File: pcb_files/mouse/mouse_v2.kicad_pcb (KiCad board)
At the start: 2 copper layers, 84.9 x 94.9 mm, 58 parts, among them J4 I2C_Conn, M1 Motor_DC, M2 Motor_DC, Q0 Q_Photo_NPN, Q1 Q_Photo_NPN, Q2 Q_Photo_NPN, Q3 Q_Photo_NPN, T0 Q_NMOS_DGS, T1 Q_NMOS_DGS, T2 Q_NMOS_DGS, T3 Q_NMOS_DGS, U1 Teensy4.0, U2 SN754410NE (Half-Bridge), U3 LM1085-5.0, U4 Encoder_3081, U5 Encoder_3081

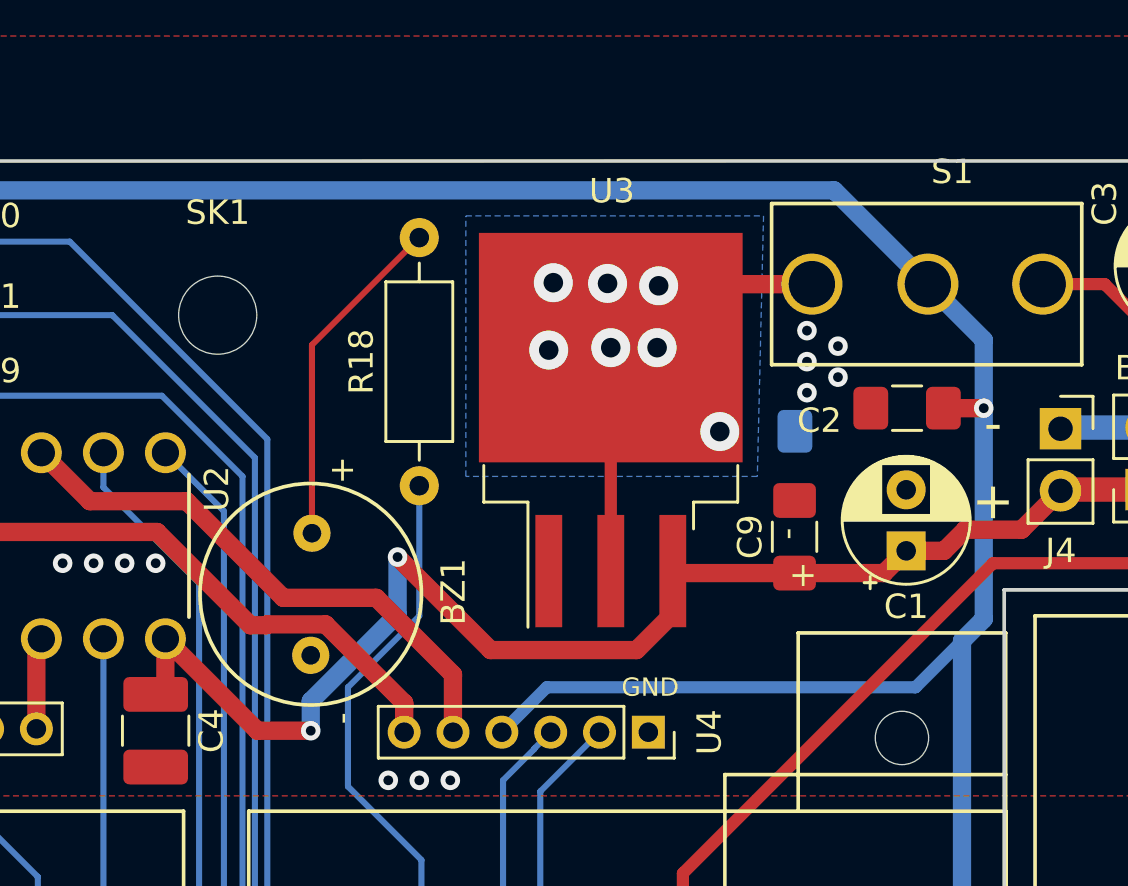
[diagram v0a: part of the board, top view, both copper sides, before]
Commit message: Silkscreen changes
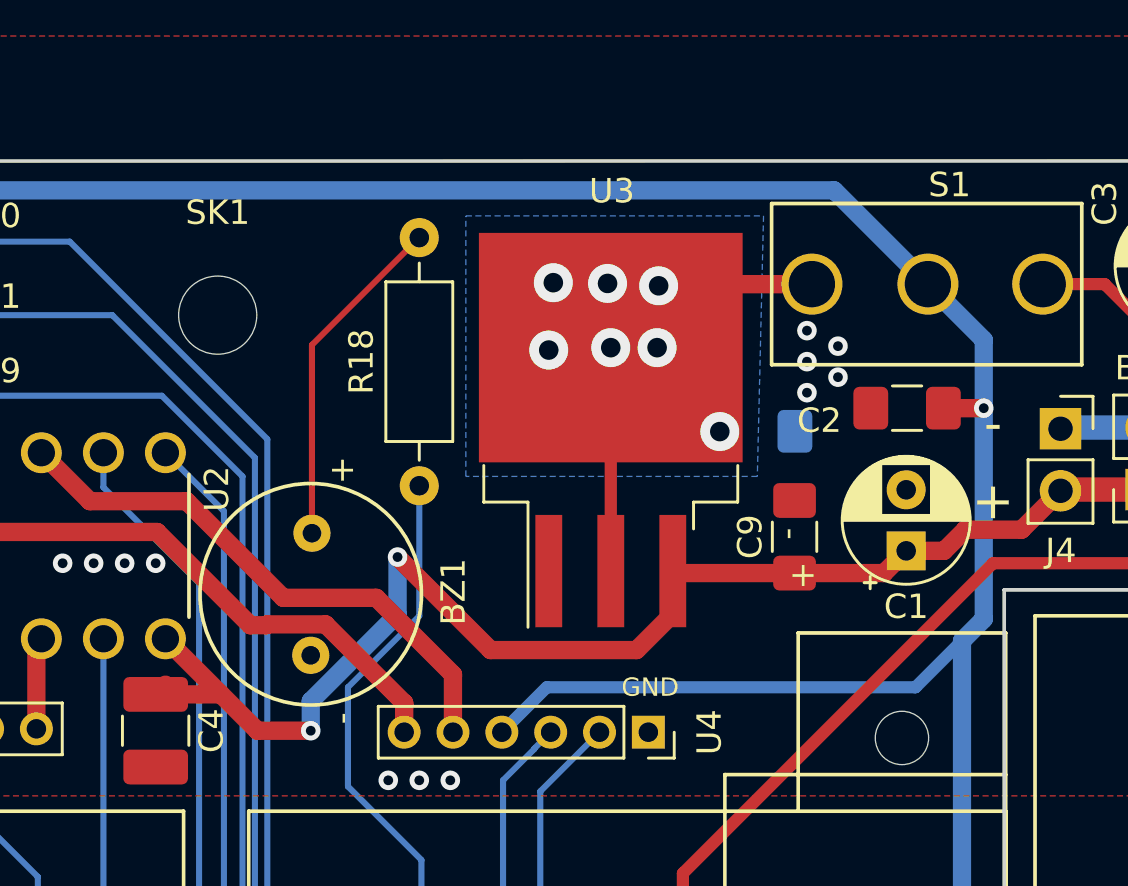
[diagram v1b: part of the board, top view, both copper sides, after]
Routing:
- net /vBatt: track 66.6 -> 67.4 mm
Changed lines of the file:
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@@
     (thickness 1.6)
     (drawings 64)
-    (tracks 429)
+    (tracks 431)
     (zones 0)
     (modules 58)
@@
   )
   (setup
-    (last_trace_width 0.13)
+    (last_trace_width 0.75)
     (user_trace_width 0.13)
     (user_trace_width 0.25)
@@
   (module misc:SWITCH_SLIDE_500SSP1S2M2QEA (layer F.Cu)
     (at 184.404 59.69)
-    (fp_text reference S1 (at 5.7 -4.6) (layer F.SilkS)
+    (fp_text reference S1 (at 5.588 -4.064) (layer F.SilkS)
       (effects (font (size 1 1) (thickness 0.15)))
     )
@@
   (segment (start 167.386 70.866) (end 167.386 73.209162) (width 0.75) (layer B.Cu) (net 1))
   (segment (start 167.386 73.209162) (end 163.83 76.765162) (width 0.75) (layer B.Cu) (net 1))
-  (segment (start 161.64306 77.978) (end 157.87878 74.21372) (width 0.75) (layer F.Cu) (net 1))
   (segment (start 163.83 77.978) (end 161.64306 77.978) (width 0.75) (layer F.Cu) (net 1))
   (segment (start 157.87878 76.09172) (end 157.48 76.4905) (width 0.75) (layer F.Cu) (net 1))
-  (segment (start 157.87878 74.21372) (end 157.87878 76.09172) (width 0.75) (layer F.Cu) (net 1))
+  (segment (start 160.08256 76.4905) (end 160.11906 76.454) (width 0.75) (layer F.Cu) (net 1))
+  (segment (start 157.48 76.4905) (end 160.08256 76.4905) (width 0.75) (layer F.Cu) (net 1))
+  (segment (start 161.64306 77.978) (end 160.11906 76.454) (width 0.75) (layer F.Cu) (net 1))
+  (segment (start 160.11906 76.454) (end 157.87878 74.21372) (width 0.75) (layer F.Cu) (net 1))
   (segment (start 194.58432 65.56248) (end 194.53352 65.61328) (width 1) (layer B.Cu) (net 2) (status 30))
   (segment (start 198.03872 65.56248) (end 194.58432 65.56248) (width 1) (layer B.Cu) (net 2) (status 30))
